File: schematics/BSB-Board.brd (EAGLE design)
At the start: 29.7 x 53.3 mm, 18 parts, among them Q1 BC107, X1 SSW-106-02-S-S, X2 SSW-116-02-S-S

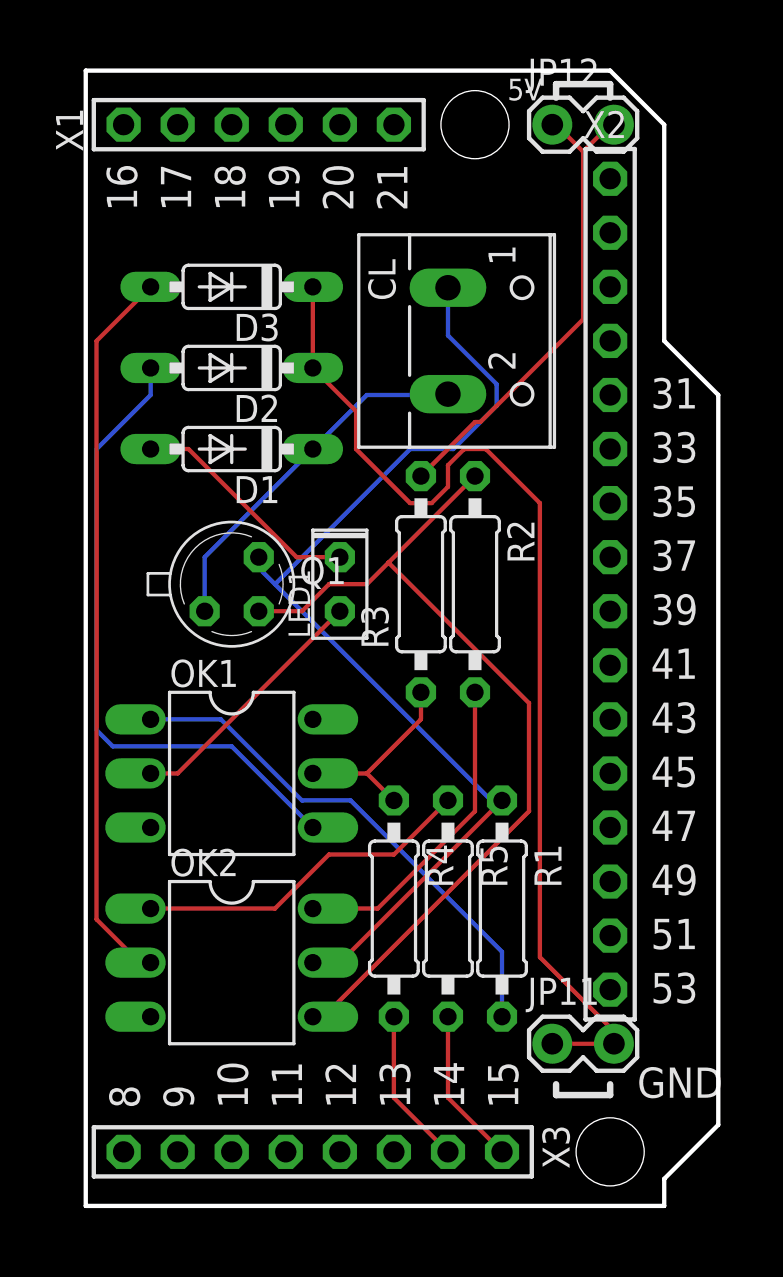
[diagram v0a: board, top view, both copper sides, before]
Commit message: New schematics for Arduino/Raspberry board
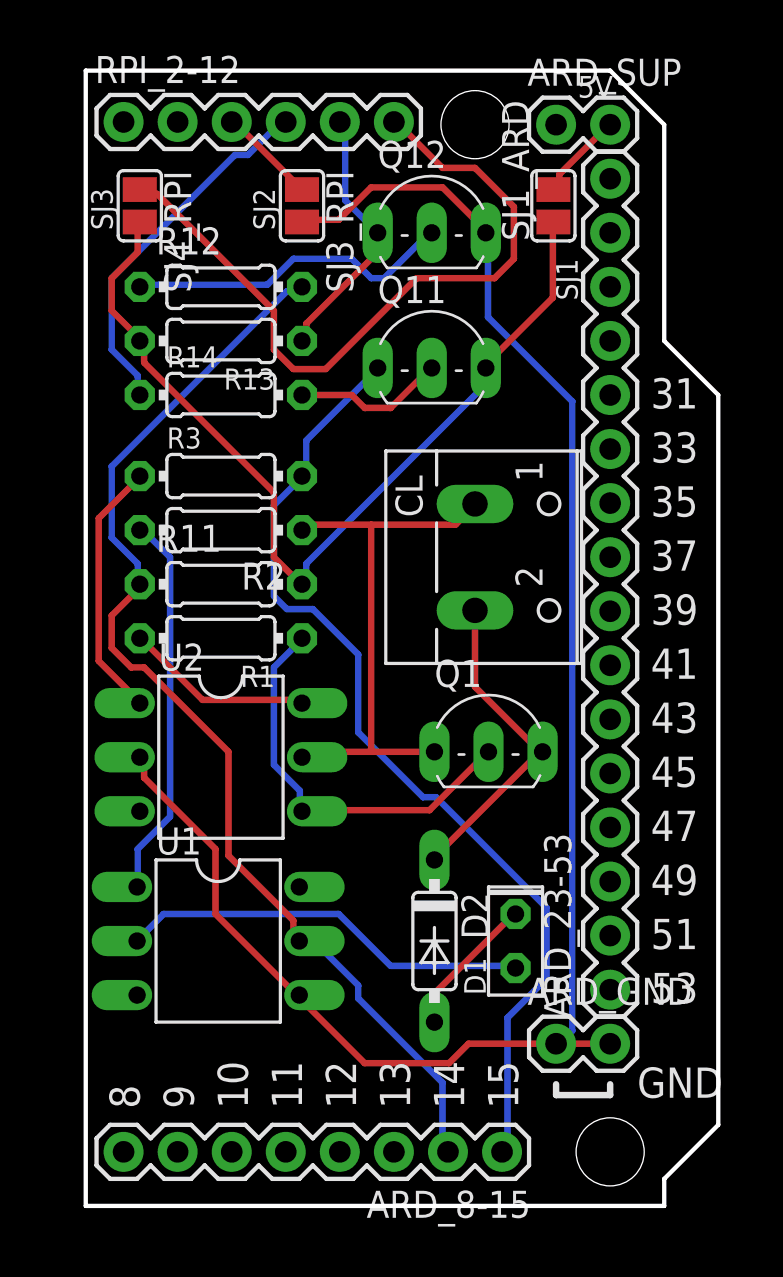
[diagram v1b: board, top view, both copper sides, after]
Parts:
- removed D3: 1N4148, diode:DO35-7
- removed JP11, JP12: (no value), SparkFun:1X02_LOCK
- removed LED1: LED->|, led:LED2X5
- removed OK1, OK2: 4N25M, optocoupler:DIL06
- removed R4: 287, eagle-ltspice:0207/10
- removed R5: 374, eagle-ltspice:0207/10
- removed X1: SSW-106-02-S-S, con-samtec:SSW-106-02-S-S
- removed X2: SSW-116-02-S-S, con-samtec:SSW-116-02-S-S
- removed X3: (no value), con-samtec:SSW-108-02-S-S
- added ARD_23-53: (no value), SparkFun-Connectors:1X16
- added ARD_8-15: (no value), SparkFun-Connectors:1X08_ROUND
- added ARD_GND, ARD_SUP: (no value), SparkFun-Connectors:1X02
- added Q11: BC 557A, transistor-neu-to92:TO92-CBE
- added Q12: BC 547A, transistor:TO92-CBE
- added R11: 4k7, resistor:0204/7
- added R12: 47k, resistor:0204/7
- added R13, R14: 10k, resistor:0204/7
- added RPI_2-12: (no value), SparkFun-Connectors:1X06
- added SJ1_ARD: Close for Arduino, jumper:SJ
- added SJ3_RPI, SJ4_RPI: Close for RPi, jumper:SJ
- added U1, U2: 4N25, optocoupler:DIL06
- CL: value - CL + -> (none)
- D1: value 1N4148 -> LED->|; device diode:DO35-7 -> led:LED2X5
- Q1: value BC107 -> BC 547A; device transistor-npn:TO18 -> transistor:TO92-CBE
- R1: value 1k5 -> 560k; device eagle-ltspice:0207/10 -> resistor:0204/7
- R2: value 560k -> 1k5; device eagle-ltspice:0207/10 -> resistor:0204/7
- R3: value 2k2 -> 300; device eagle-ltspice:0207/10 -> resistor:0204/7
- moved D2 28.6 mm to (16.4, 12.4), turned to 270 degrees
- moved D1 26.7 mm to (20.2, 12.4), turned to 90 degrees
- moved R1 18.3 mm to (6.35, 26.7), turned to 180 degrees
- moved Q1 14.4 mm to (18.9, 21.3)
- moved R2 12.2 mm to (6.35, 31.8), turned to 180 degrees
- moved R3 10.7 mm to (6.35, 34.3), turned to 0 degrees
- moved CL 10.2 mm to (19.6, 30.5)
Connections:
- removed net A14: R4.2, X3.2
- removed net A15: R5.2, X3.1
- removed net D23: X2.1
- removed net D25: X2.2
- removed net D27: X2.3
- removed net D29: X2.4
- removed net D31: X2.5
- removed net D33: X2.6
- removed net D35: X2.7
- removed net D37: X2.8
- removed net D39: X2.9
- removed net D41: X2.10
- removed net D43: X2.11
- removed net D45: X2.12
- removed net D47: X2.13
- removed net D49: X2.14
- removed net D51: X2.15
- removed net D53: X2.16
- removed net N$10: D2.C, D3.C, JP11.1, JP11.2
- removed net N$13: D3.A, OK2.2
- removed net N$14: JP12.1, JP12.2, R3.2
- removed net N$7: CL.2, D1.C, Q1.1
- removed net N$8: OK1.5, R3.1, R4.1
- new net 5V-ARD: ARD_SUP.2, SJ1_ARD.2
- new net A14-RXD-ARD: ARD_8-15.2, R11.1, R12.2, U1.5
- new net A15-TXD-ARD: ARD_8-15.1, Q11.C, R3.2
- new net CL+: CL.1, Q1.C, R2.1, U2.5
- new net CL-: CL.2, D2.C, Q1.E
- new net GND-ARD: ARD_GND.1, ARD_GND.2, Q12.E, SJ3_RPI.2, U1.4, U2.2
- new net GPIO14-TXD-PI: R14.1, RPI_2-12.4
- new net GPIO15-RXD-PI: Q12.C, R13.1, RPI_2-12.5
- new net GPIO18-3V3-PI: RPI_2-12.6, SJ4_RPI.1
- new net PIN6-GND-PI: RPI_2-12.3, SJ3_RPI.1
- new net VCC: Q11.E, R11.2, R13.2, SJ1_ARD.1, SJ4_RPI.2
- net N$1: now also R2.2, U1.1; no longer OK1.1, R1.2
- net N$11: now also R3.1, U2.1; no longer OK2.1, R5.1
- net N$2: now also D1.A, U1.2; no longer LED1.A, OK1.2
- net N$3: now also R1.2, U2.6; no longer OK2.6, R2.2
- net N$4: now also D1.K, D2.A; no longer D1.A, LED1.K
- net N$5: now also Q1.B, R1.1, U2.4; no longer OK2.4, Q1.2, R2.1
- net N$6: now also Q12.B, R12.1; no longer CL.1, OK2.5, Q1.3, R1.1
- net N$9: now also Q11.B, R14.2; no longer D2.A, OK1.4
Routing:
- net GND-ARD: track 0.00 -> 81.4 mm
- net A14-RXD-ARD: track 0.00 -> 53.3 mm
- net N$10: track 50.5 -> 0.00 mm
- net A15-TXD-ARD: track 0.00 -> 46.1 mm
- net VCC: track 0.00 -> 43.3 mm
- net N$13: track 34.2 -> 0.00 mm
- net GPIO18-3V3-PI: track 0.00 -> 34.0 mm
- net N$6: track 48.9 -> 15.5 mm
- net CL+: track 0.00 -> 25.7 mm
- net N$9: track 30.1 -> 7.12 mm
- net N$14: track 22.5 -> 0.00 mm
- net N$5: track 41.4 -> 19.1 mm
- net GPIO14-TXD-PI: track 0.00 -> 17.3 mm
- net N$7: track 17.2 -> 0.00 mm
- net CL-: track 0.00 -> 15.1 mm
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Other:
- board text added: "Arduino Connector RX TX"
- board text added: "DB CL+"
- board text added: "MB CL-"
- board text added: "RX"
- board text added: "RasPi 06 08 10 12"
- board text added: "SJ1"
- board text added: "SJ2"
- board text added: "SJ3"
- board text added: "Schematics by G.Schumacher / J.Loehnert Board layout by Frederik Holst"
- board text added: "Solder Jumpers: Arduino: connect SJ1 (5V) Raspi: connect SJ2 (GND) and S3 (3.3V)"
- board text added: "TX"
- board text removed: "16"
- board text removed: "17"
- board text removed: "18"
- board text removed: "19"
- board text removed: "20"
- board text removed: "21"
- board text removed: "Schematics by Gero Schumacher Board layout by Frederik Holst"
